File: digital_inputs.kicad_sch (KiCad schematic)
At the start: 182 parts, among them J1 6437288-2, J10 Conn_01x01, J11 Conn_01x01, J12 Conn_01x01, J13 Conn_01x01, J14 Conn_01x01, J15 Conn_01x01, J16 Conn_01x01, J17 Conn_01x01, J19 6437288-3, J20 Conn_02x10_Odd_Even, J21 Conn_02x08_Odd_Even, J22 Conn_02x15_Odd_Even, J23 Conn_02x10_Odd_Even, J24 Conn_02x17_Odd_Even, J25 Conn_02x10_Odd_Even, J26 Conn_02x06_Odd_Even, J27 Conn_02x16_Odd_Even, J28 Conn_02x04_Odd_Even, J29 Conn_02x10_Odd_Even, J3 Conn_01x08, J30 Conn_02x14_Odd_Even, J4 Conn_01x01, J5 Conn_01x02, J6 Conn_01x04, J7 Conn_01x04, J8 Conn_01x04, J9 Conn_01x04, P1 Pad, P10 Pad, P11 Pad, P12 Pad, P13 Pad, P14 Pad, P15 Pad, P16 Pad, P17 Pad, P18 Pad, P19 Pad, P2 Pad, P3 Pad, P4 Pad, P5 Pad, P6 Pad, P7 Pad, P8 Pad, P9 Pad, Q1 AO3400A, Q2 AO3400A, Q3 AO3400A, Q4 AO3400A, Q5 AO3400A, Q6 AO3400A, Q7 AO3400A, Q8 AO3400A, U1 OPA2192IDR, U10 ULN2003A, U11 OPA2192IDR, U12 TJA1051T-3, U13 TJA1051T-3, U14 LM78M05_TO252, U2 CD4067BM96, U3 CD4067BM96, U4 CD4067BM96, U5 CD4067BM96, U6 CD4067BM96, U7 CD4067BM96, U8 TC4427, U9 TC4427

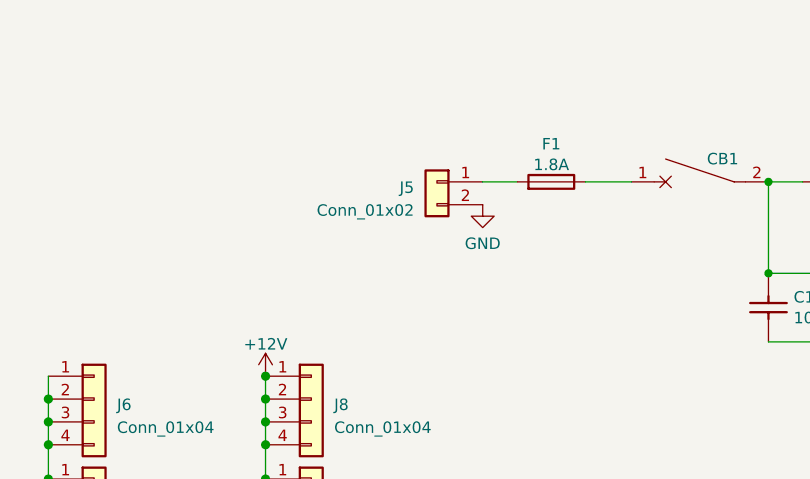
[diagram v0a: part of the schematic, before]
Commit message: #52
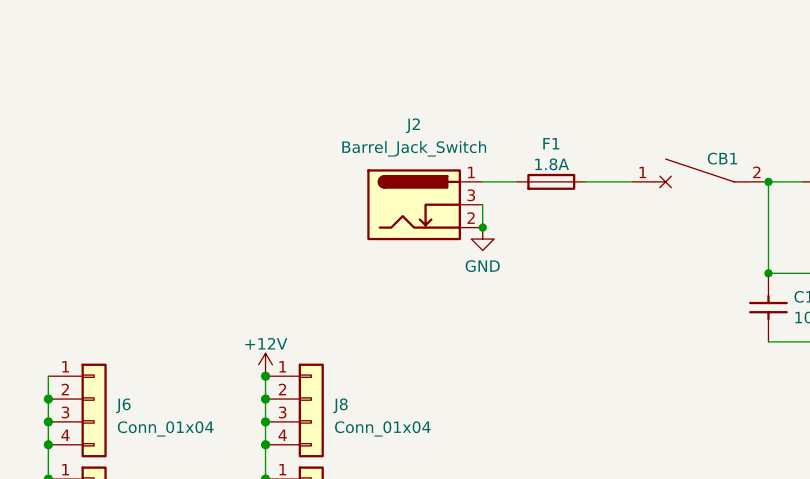
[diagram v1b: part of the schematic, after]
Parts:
- removed J5: Conn_01x02, TerminalBlock_Phoenix:TerminalBlock_Phoenix_MKDS-1,5-2-5.08_1x02_P5.08mm_Horizontal, symbol Connector_Generic:Conn_01x02
- added J2: Barrel_Jack_Switch, Connector_BarrelJack:BarrelJack_GCT_DCJ200-10-A_Horizontal, symbol Connector:Barrel_Jack_Switch
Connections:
- net GND: now also J2.2, J2.3
- net at F1.2: now also J2.1
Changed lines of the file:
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@@
 	)
 	(junction
+		(at 369.57 43.18)
+		(diameter 0)
+		(color 0 0 0 0)
+	)
+	(junction
 		(at 345.44 73.66)
 		(diameter 1.016)
@@
 	(wire
 		(pts
+			(xy 369.57 43.18) (xy 369.57 40.64)
+		)
+		(stroke
+			(width 0)
+			(type default)
+		)
+	)
+	(wire
+		(pts
 			(xy 231.14 99.06) (xy 241.3 99.06)
 		)
@@
 	)
 	(symbol
+		(lib_id "Connector:Barrel_Jack_Switch")
+		(at 361.95 40.64 0)
+		(unit 1)
+		(exclude_from_sim no)
+		(in_bom yes)
+		(on_board yes)
+		(dnp no)
+		(fields_autoplaced yes)
+		(property "Reference" "J2"
+			(at 361.95 31.75 0)
+			(effects
+				(font
+					(size 1.27 1.27)
+				)
+			)
+		)
+		(property "Value" "Barrel_Jack_Switch"
+			(at 361.95 34.29 0)
+			(effects
+				(font
+					(size 1.27 1.27)
+				)
+			)
+		)
+		(property "Footprint" "Connector_BarrelJack:BarrelJack_GCT_DCJ200-10-A_Horizontal"
+			(at 363.22 41.656 0)
+			(effects
+				(font
+					(size 1.27 1.27)
+				)
+				(hide yes)
+			)
+		)
+		(property "Datasheet" "~"
+			(at 363.22 41.656 0)
+			(effects
+				(font
+					(size 1.27 1.27)
+				)
+				(hide yes)
+			)
+		)
+		(property "Description" "DC Barrel Jack with an internal switch"
+			(at 361.95 40.64 0)
+			(effects
+				(font
+					(size 1.27 1.27)
+				)
+				(hide yes)
+			)
+		)
+		(property "LCSC" "C111567"
+			(at 361.95 40.64 0)
+			(effects
+				(font
+					(size 1.27 1.27)
+				)
+				(hide yes)
+			)
+		)
+		(pin "2"
+		)
+		(pin "1"
+		)
+		(pin "3"
+		)
+		(instances
+			(project ""
+				(path "/4c34721c-e264-4f09-9eef-002c922c83d1"
+					(reference "J2")
+					(unit 1)
+				)
+			)
+		)
+	)
+	(symbol
 		(lib_id "power:GND")
 		(at 408.94 361.95 270)
@@
 	(symbol
 		(lib_id "power:GND")
-		(at 369.57 40.64 0)
+		(at 369.57 43.18 0)
 		(unit 1)
 		(exclude_from_sim no)
@@
 		(fields_autoplaced yes)
 		(property "Reference" "#PWR02"
-			(at 369.57 46.99 0)
+			(at 369.57 49.53 0)
 			(effects
 				(font
@@
 		)
 		(property "Value" "GND"
-			(at 369.57 44.9644 0)
+			(at 369.57 47.5044 0)
 			(effects
 				(font
@@
 		)
 		(property "Footprint" ""
-			(at 369.57 40.64 0)
+			(at 369.57 43.18 0)
 			(effects
 				(font
@@
 		)
 		(property "Datasheet" ""
-			(at 369.57 40.64 0)
+			(at 369.57 43.18 0)
 			(effects
 				(font
@@
 		)
 		(property "Description" ""
-			(at 369.57 40.64 0)
+			(at 369.57 43.18 0)
 			(effects
 				(font
@@
 					(unit 1)
 				)
-			)
-		)
-	)
-	(symbol
-		(lib_id "Connector_Generic:Conn_01x02")
-		(at 364.49 38.1 0)
-		(mirror y)
-		(unit 1)
-		(exclude_from_sim no)
-		(in_bom yes)
-		(on_board yes)
-		(dnp no)
-		(fields_autoplaced yes)
-		(property "Reference" "J5"
-			(at 361.95 38.7349 0)
-			(effects
-				(font
-					(size 1.27 1.27)
-				)
-				(justify left)
-			)
-		)
-		(property "Value" "Conn_01x02"
-			(at 361.95 41.2749 0)
-			(effects
-				(font
-					(size 1.27 1.27)
-				)
-				(justify left)
-			)
-		)
-		(property "Footprint" "TerminalBlock_Phoenix:TerminalBlock_Phoenix_MKDS-1,5-2-5.08_1x02_P5.08mm_Horizontal"
-			(at 364.49 38.1 0)
-			(effects
-				(font
-					(size 1.27 1.27)
-				)
-				(hide yes)
-			)
-		)
-		(property "Datasheet" "~"
-			(at 364.49 38.1 0)
-			(effects
-				(font
-					(size 1.27 1.27)
-				)
-				(hide yes)
-			)
-		)
-		(property "Description" ""
-			(at 364.49 38.1 0)
-			(effects
-				(font
-					(size 1.27 1.27)
-				)
-				(hide yes)
-			)
-		)
-		(pin "1"
-		)
-		(pin "2"
-		)
-		(instances
-			(project "digital_inputs"
-				(path "/4c34721c-e264-4f09-9eef-002c922c83d1"
-					(reference "J5")
-					(unit 1)
-				)
